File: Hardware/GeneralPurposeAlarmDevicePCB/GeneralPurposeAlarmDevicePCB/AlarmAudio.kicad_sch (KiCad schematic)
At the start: 12 parts, among them J601 22-23-2021, Q601 MMBT2222A-7-F, Q602 MMBT2907ALT1G

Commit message: updated buzzer footprint to a generic compatible one
Signed-off-by: lokimetasmith <lokimail@gmail.com>
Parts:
- BZ601: footprint QMB-09B-03:QMB09B03 -> Buzzer_Beeper:MagneticBuzzer_PUI_AT-0927-TT-6-R
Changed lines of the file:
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@@
     (property "Reference" "BZ601" (id 0) (at 197.9168 99.441 0))
     (property "Value" "QMB-09B-03" (id 1) (at 197.9168 97.1296 0))
-    (property "Footprint" "QMB-09B-03:QMB09B03" (id 2) (at 189.865 87.63 90)
+    (property "Footprint" "Buzzer_Beeper:MagneticBuzzer_PUI_AT-0927-TT-6-R" (id 2) (at 189.865 87.63 90)
       (effects (font (size 1.27 1.27)) hide)
     )

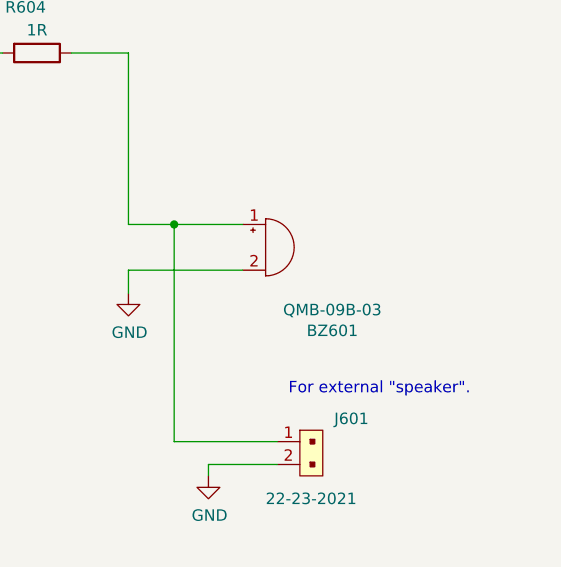
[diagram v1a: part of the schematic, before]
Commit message: Update buzzer foot print. Fully connect all parts. Fix numerous silkscreen conflicts. Mix of metric and imperial grid.
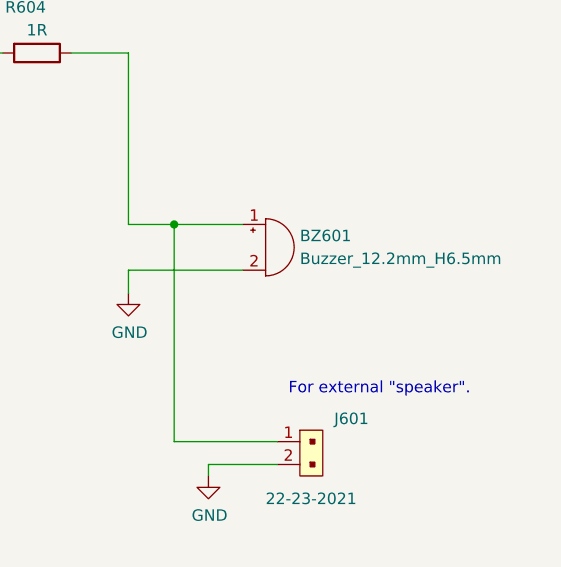
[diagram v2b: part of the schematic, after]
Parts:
- BZ601: value QMB-09B-03 -> Buzzer_12.2mm_H6.5mm; footprint Buzzer_Beeper:MagneticBuzzer_PUI_AT-0927-TT-6-R -> Buzzer_Beeper:Buzzer_TDK_PS1240P02BT_D12.2mm_H6.5mm; Cost (none) -> 0.62000; Distributor 1 PN C96256 -> C76871; Distributor 2 (none) -> Digi-Key; Distributor 2 PN (none) -> 445-2525-1-ND; MPN QMB-09B-03 -> PS1240P02BT; Manufacturer Jiangsu Huaneng Elec -> TDK Corporation
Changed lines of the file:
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@@
-    (pin "2")
-  )
-  (symbol (lib_id "Device:Buzzer") (at 190.5 90.17 0) (unit 1)
-    (in_bom yes) (on_board yes)
-    (property "Reference" "BZ601" (id 0) (at 197.9168 99.441 0))
-    (property "Value" "QMB-09B-03" (id 1) (at 197.9168 97.1296 0))
-    (property "Footprint" "Buzzer_Beeper:MagneticBuzzer_PUI_AT-0927-TT-6-R" (id 2) (at 189.865 87.63 90)
-      (effects (font (size 1.27 1.27)) hide)
-    )
-    (property "Datasheet" "~" (id 3) (at 189.865 87.63 90)
-      (effects (font (size 1.27 1.27)) hide)
-    )
-    (property "Description" "Magnetic NO 2700Hz 3V 2 ~ 5V 9mm 9*5.5mm Buzzers" (id 4) (at 207.01 92.71 0)
-      (effects (font (size 1.27 1.27)) (justify left) hide)
-    )
-    (property "Manufacturer" "Jiangsu Huaneng Elec" (id 5) (at 207.01 97.79 0)
-      (effects (font (size 1.27 1.27)) (justify left) hide)
-    )
-    (property "MPN" "QMB-09B-03" (id 6) (at 207.01 100.33 0)
-      (effects (font (size 1.27 1.27)) (justify left) hide)
-    )
-    (property "Distributor 1" "JLCPCB" (id 7) (at 190.5 90.17 0)
-      (effects (font (size 1.27 1.27)) hide)
-    )
-    (property "Distributor 1 PN" "C96256" (id 8) (at 190.5 90.17 0)
-      (effects (font (size 1.27 1.27)) hide)
-    )
-    (pin "1")
     (pin "2")
   )
@@
       (effects (font (size 1.27 1.27)) hide)
     )
+    (pin "1")
+    (pin "2")
+  )
+  (symbol (lib_id "Device:Buzzer") (at 190.5 90.17 0) (unit 1)
+    (in_bom yes) (on_board yes) (fields_autoplaced)
+    (property "Reference" "BZ601" (id 0) (at 194.31 88.8999 0)
+      (effects (font (size 1.27 1.27)) (justify left))
+    )
+    (property "Value" "Buzzer_12.2mm_H6.5mm" (id 1) (at 194.31 91.4399 0)
+      (effects (font (size 1.27 1.27)) (justify left))
+    )
+    (property "Footprint" "Buzzer_Beeper:Buzzer_TDK_PS1240P02BT_D12.2mm_H6.5mm" (id 2) (at 189.865 87.63 90)
+      (effects (font (size 1.27 1.27)) hide)
+    )
+    (property "Datasheet" "~" (id 3) (at 189.865 87.63 90)
+      (effects (font (size 1.27 1.27)) hide)
+    )
+    (property "Distributor 1" "JLCPCB" (id 9) (at 190.5 90.17 0)
+      (effects (font (size 1.27 1.27)) hide)
+    )
+    (property "Distributor 1 PN" "C76871" (id 10) (at 190.5 90.17 0)
+      (effects (font (size 1.27 1.27)) hide)
+    )
+    (property "Distributor 2" "Digi-Key" (id 5) (at 190.5 90.17 0)
+      (effects (font (size 1.27 1.27)) hide)
+    )
+    (property "Distributor 2 PN" "445-2525-1-ND" (id 6) (at 190.5 90.17 0)
+      (effects (font (size 1.27 1.27)) hide)
+    )
+    (property "Manufacturer" "TDK Corporation" (id 7) (at 190.5 90.17 0)
+      (effects (font (size 1.27 1.27)) hide)
+    )
+    (property "MPN" "PS1240P02BT" (id 8) (at 190.5 90.17 0)
+      (effects (font (size 1.27 1.27)) hide)
+    )
+    (property "Cost" "0.62000" (id 9) (at 190.5 90.17 0)
+      (effects (font (size 1.27 1.27)) hide)
+    )
